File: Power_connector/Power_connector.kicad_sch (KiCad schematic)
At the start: 52 parts, among them J1 XT60_F, J10 XT60_F, J11 XT60_F, J12 XT60_F, J13 XT60_F, J14 XT60_F, J2 XT60_Male, J3 XT60_F, J4 XT60_F, J5 Screw_Terminal_01x02, J6 XT60_F, J7 XT60_F, J8 XT60_F, J9 XT60_F, Q1 IRFS7530, Q2 IRFS7530, Q3 IRFS7530, Q4 IRFS7530

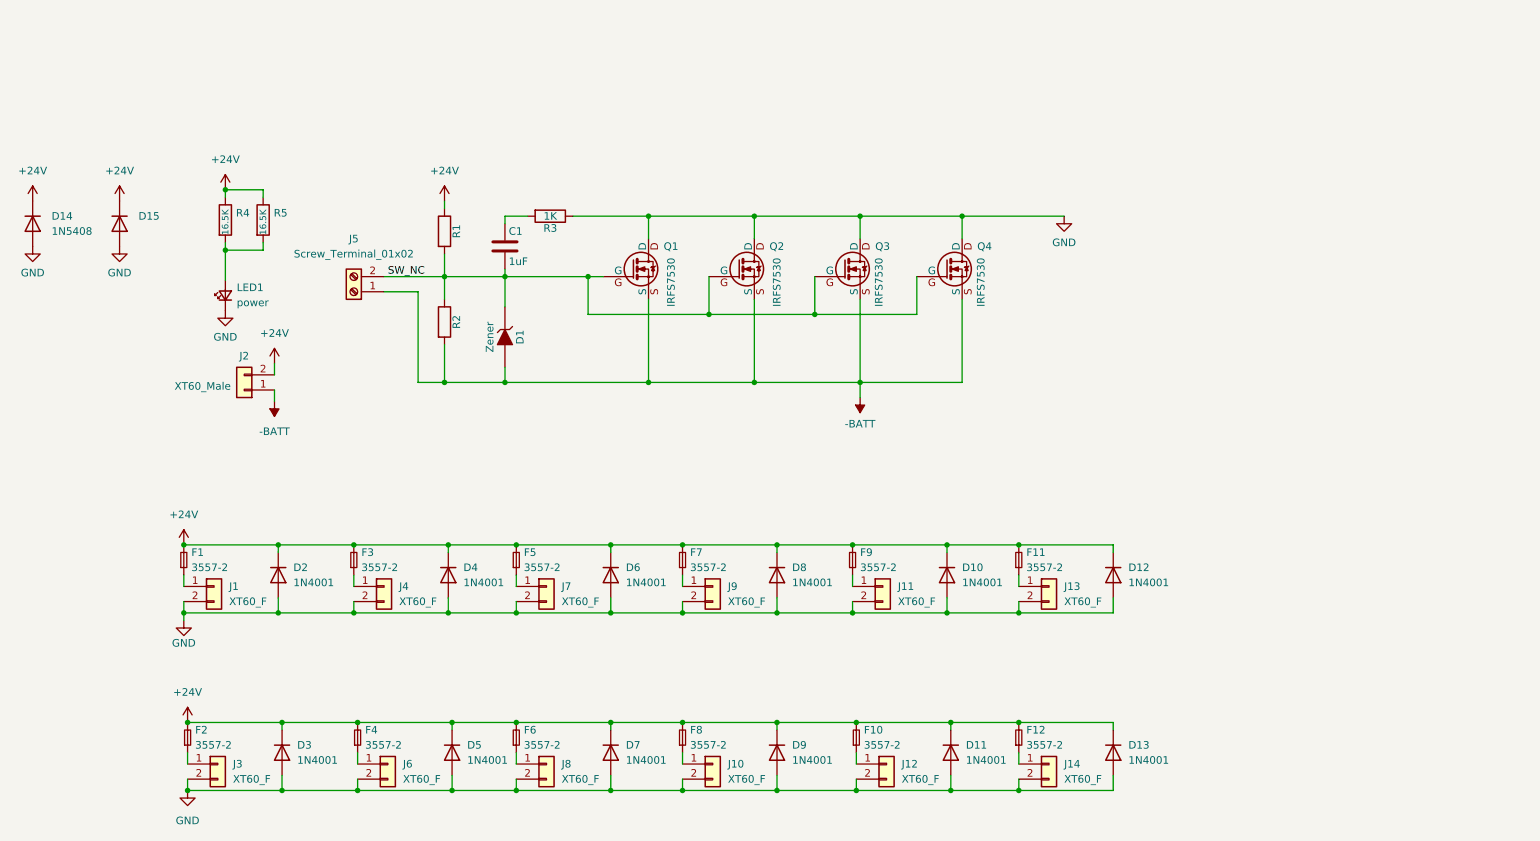
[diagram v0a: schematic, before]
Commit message: powerboard mod
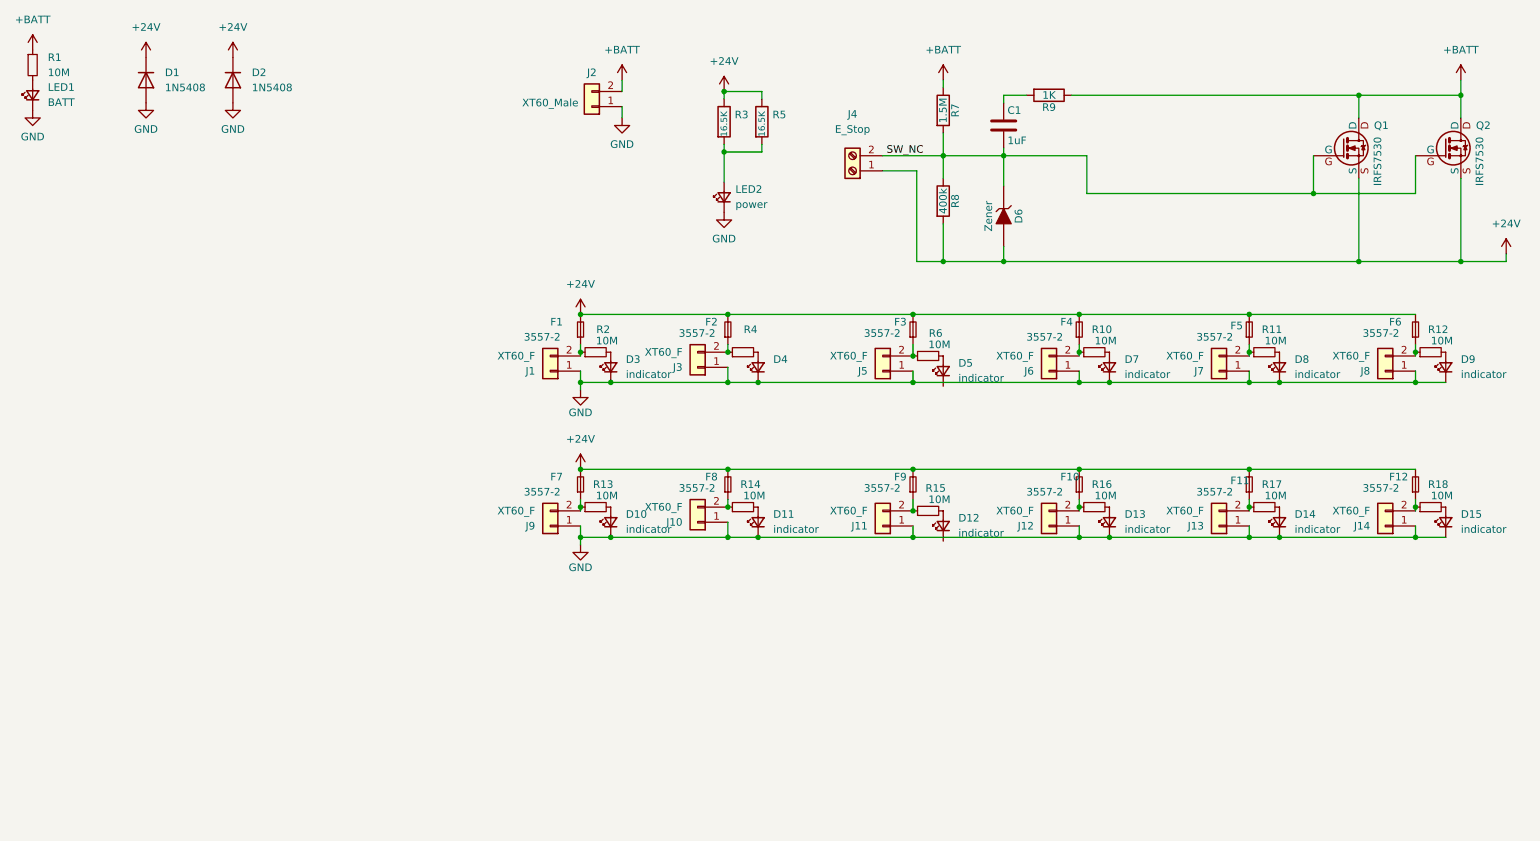
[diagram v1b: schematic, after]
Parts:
- removed D10, D11, D12, D13, D2, D3, D4, D5, D6, D7, D8, D9: 1N4001, Diode_THT:D_DO-41_SOD81_P10.16mm_Horizontal, symbol Diode:1N4001
- removed F2, F4, F6: 3557-2, PolyuRobotics:FUSE_3557-2, symbol Device:Fuse_Small
- removed J3, J6, J8: XT60_F, Connector_AMASS:AMASS_XT60-F_1x02_P7.20mm_Vertical, symbol Connector_Generic:Conn_01x02
- removed Q1, Q2: IRFS7530, sparkparts:D2PAK-7-GDS, symbol sparkparts:IRFS7530
- added D10, D11, D12, D13, D14, D15, D3, D5, D7, D8, D9: indicator, symbol Device:LED_Small
- added D4: (no value), symbol Device:LED_Small
- added F11, F7, F9: 3557-2, PolyuRobotics:FUSE_3557-2, symbol Device:Fuse_Small
- added J11, J13, J9: XT60_F, Connector_AMASS:AMASS_XT60-F_1x02_P7.20mm_Vertical, symbol Connector_Generic:Conn_01x02
- added LED1: BATT, LED_SMD:LED_0805_2012Metric_Pad1.15x1.40mm_HandSolder, symbol Device:LED_Small
- added R1: 10M, Resistor_SMD:R_0805_2012Metric, symbol Device:R_Small
- added R10, R11, R12, R13, R14, R15, R16, R17, R18, R2, R6: 10M, symbol Device:R_Small
- added R4: (no value), symbol Device:R_Small
- D2: renamed from D15; value (none) -> 1N5408; footprint (none) -> Diode_THT:D_DO-201AD_P15.24mm_Horizontal
- J4: renamed from J5; value Screw_Terminal_01x02 -> E_Stop
- R7: renamed from R1; value (none) -> 1.5M
- R8: renamed from R2; value (none) -> 400k
- renumbered D14 to D1, D1 to D6, F3 to F2, F5 to F3, F7 to F4, F9 to F5, F11 to F6, J4 to J3, J7 to J5, J9 to J6, J11 to J7, J13 to J8, LED1 to LED2, Q3 to Q1, Q4 to Q2, R4 to R3, R3 to R9
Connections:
- net +24V: now also D6.2 (A), J4.1 (Pin_1), Q1.S, Q2.S, R8.2, F11.2, F7.2, F9.2; no longer J2.2 (Pin_2), R7.1
- net GND: now also J1.1 (Pin_1), J10.1 (Pin_1), J12.1 (Pin_1), J14.1 (Pin_1), J2.1 (Pin_1), J3.1 (Pin_1), J5.1 (Pin_1), J6.1 (Pin_1), J7.1 (Pin_1), J8.1 (Pin_1), D10.1 (K), D11.1 (K), D13.1 (K), D14.1 (K), D15.1 (K), D3.1 (K), D4.1 (K), D7.1 (K), D8.1 (K), D9.1 (K), J11.1 (Pin_1), J13.1 (Pin_1), J9.1 (Pin_1), LED1.1 (K); no longer J1.2 (Pin_2), J10.2 (Pin_2), J12.2 (Pin_2), J14.2 (Pin_2), J3.2 (Pin_2), J5.2 (Pin_2), J6.2 (Pin_2), J7.2 (Pin_2), J8.2 (Pin_2), Q1.D, Q2.D, R9.1
- net at F2.1: now also J3.2 (Pin_2), R4.1; no longer J3.1 (Pin_1)
- net at F10.1: now also J12.2 (Pin_2), R16.1; no longer J12.1 (Pin_1)
- net at F8.1: now also J10.2 (Pin_2), R14.1; no longer J10.1 (Pin_1)
- net at F4.1: now also J6.2 (Pin_2), R10.1; no longer J6.1 (Pin_1)
- net at F1.1: now also J1.2 (Pin_2), R2.1; no longer J1.1 (Pin_1)
- net at F5.1: now also J7.2 (Pin_2), R11.1; no longer J7.1 (Pin_1)
- net at F12.1: now also J14.2 (Pin_2), R18.1; no longer J14.1 (Pin_1)
- net at F6.1: now also J8.2 (Pin_2), R12.1; no longer J8.1 (Pin_1)
- net at F3.1: now also J5.2 (Pin_2), R6.1; no longer J5.1 (Pin_1)
- removed net -BATT: D6.2 (A), J2.1 (Pin_1), J4.1 (Pin_1), Q1.S, Q2.S, R8.2
- new net: LED1.2 (A), R1.2
- new net: D3.2 (A), R2.2
- new net: D7.2 (A), R10.2
- new net: D8.2 (A), R11.2
- new net: F7.1, J9.2 (Pin_2), R13.1
- new net: D13.2 (A), R16.2
- new net: D12.2 (A), R15.2
- new net: D10.2 (A), R13.2
- new net: D15.2 (A), R18.2
- new net: F9.1, J11.2 (Pin_2), R15.1
- new net: F11.1, J13.2 (Pin_2), R17.1
- new net: D4.2 (A), R4.2
- new net: D5.2 (A), R6.2
- new net: D9.2 (A), R12.2
- new net: D14.2 (A), R17.2
- new net: D11.2 (A), R14.2
- new net +BATT: J2.2 (Pin_2), Q1.D, Q2.D, R1.1, R7.1, R9.1
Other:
- moved on the sheet: C1, D1, D2, D6, F1, F2, F3, F4, F5, F6, J1, J2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
